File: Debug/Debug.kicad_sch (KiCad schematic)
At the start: 37 parts, among them J1 Expansion_Connector, SW1 Step, SW2 PHI1/Step, SW3 Run, SW4 SI/SC, U1 74HCT04, U10 MC14495P1, U11 HDSP-7803, U12 MC14495P1, U13 HDSP-7803, U14 MC14495P1, U15 HDSP-7803, U2 74HCT74, U3 MC14495P1, U4 HDSP-7803, U5 74HCT374, U6 MC14495P1, U7 HDSP-7803, U8 MC14495P1, U9 HDSP-7803

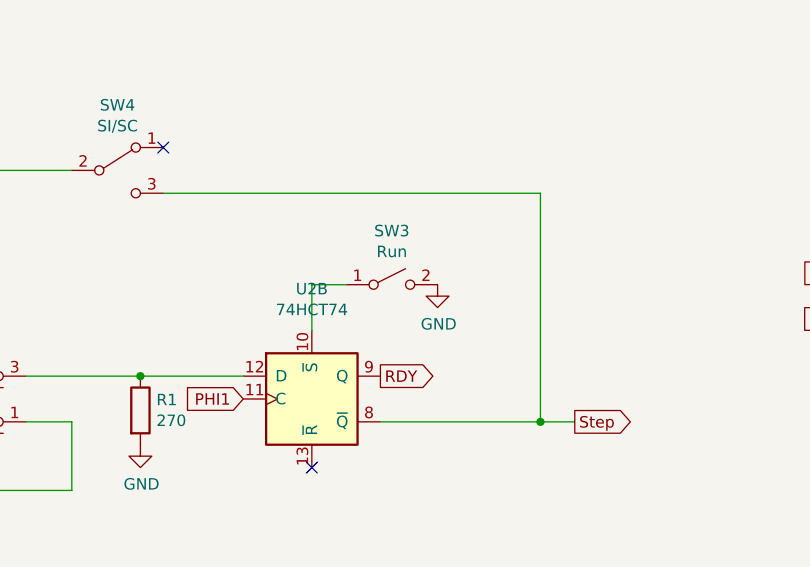
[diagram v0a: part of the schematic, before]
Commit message: Update Debug.kicad_sch
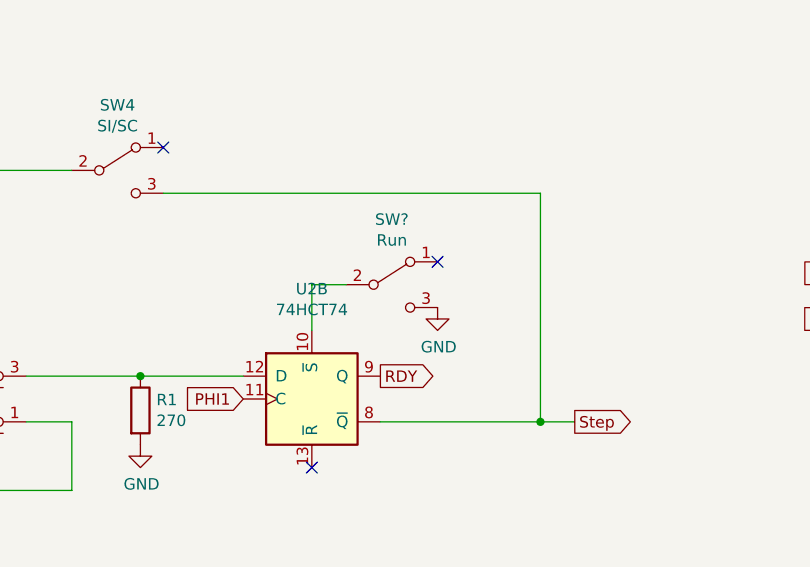
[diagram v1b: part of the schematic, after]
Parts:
- removed SW3: Run, Button_Switch_THT:SW_DIP_SPSTx01_Slide_9.78x4.72mm_W7.62mm_P2.54mm, symbol Switch:SW_SPST
- added SW?: Run, Button_Switch_THT:SW_Slide_1P2T_CK_OS102011MS2Q, symbol Switch:SW_SPDT
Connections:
- net GND: now also SW?.3 (C)
- net at U2.10 (~{S}): now also SW?.2 (B)
- no-connect marks 25 -> 26
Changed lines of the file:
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@@
   (no_connect (at 346.71 48.26))
   (no_connect (at 140.97 208.28))
+  (no_connect (at 274.32 143.51))
   (no_connect (at 233.68 46.99))
   (no_connect (at 224.79 48.26))
@@
     (pin "7")
   )
-  (symbol (lib_id "Switch:SW_SPST") (at 269.24 146.05 0) (unit 1)
-    (in_bom yes) (on_board yes)
-    (property "Reference" "SW3" (id 0) (at 269.24 140.081 0))
-    (property "Value" "Run" (id 1) (at 269.24 142.3924 0))
-    (property "Footprint" "Button_Switch_THT:SW_DIP_SPSTx01_Slide_9.78x4.72mm_W7.62mm_P2.54mm" (id 2) (at 269.24 146.05 0)
-      (effects (font (size 1.27 1.27)) hide)
-    )
-    (property "Datasheet" "~" (id 3) (at 269.24 146.05 0)
-      (effects (font (size 1.27 1.27)) hide)
-    )
-    (pin "1")
-    (pin "2")
-  )
-  (symbol (lib_id "power:GND") (at 274.32 146.05 0) (unit 1)
-    (in_bom yes) (on_board yes)
-    (property "Reference" "#PWR0104" (id 0) (at 274.32 152.4 0)
-      (effects (font (size 1.27 1.27)) hide)
-    )
-    (property "Value" "GND" (id 1) (at 274.447 150.4442 0))
-    (property "Footprint" "" (id 2) (at 274.32 146.05 0)
-      (effects (font (size 1.27 1.27)) hide)
-    )
-    (property "Datasheet" "" (id 3) (at 274.32 146.05 0)
+  (symbol (lib_id "power:GND") (at 274.32 148.59 0) (unit 1)
+    (in_bom yes) (on_board yes)
+    (property "Reference" "#PWR0104" (id 0) (at 274.32 154.94 0)
+      (effects (font (size 1.27 1.27)) hide)
+    )
+    (property "Value" "GND" (id 1) (at 274.447 152.9842 0))
+    (property "Footprint" "" (id 2) (at 274.32 148.59 0)
+      (effects (font (size 1.27 1.27)) hide)
+    )
+    (property "Datasheet" "" (id 3) (at 274.32 148.59 0)
       (effects (font (size 1.27 1.27)) hide)
     )
@@
     (pin "9")
   )
+  (symbol (lib_id "Switch:SW_SPDT") (at 269.24 146.05 0) (unit 1)
+    (in_bom yes) (on_board yes)
+    (property "Reference" "SW?" (id 0) (at 269.24 138.811 0))
+    (property "Value" "Run" (id 1) (at 269.24 141.1224 0))
+    (property "Footprint" "Button_Switch_THT:SW_Slide_1P2T_CK_OS102011MS2Q" (id 2) (at 269.24 146.05 0)
+      (effects (font (size 1.27 1.27)) hide)
+    )
+    (property "Datasheet" "~" (id 3) (at 269.24 146.05 0)
+      (effects (font (size 1.27 1.27)) hide)
+    )
+    (pin "1")
+    (pin "2")
+    (pin "3")
+  )
   (symbol (lib_id "power:GND") (at 149.86 128.27 0) (unit 1)
     (in_bom yes) (on_board yes)
@@
       (reference "SW2") (unit 1) (value "PHI1/Step") (footprint "Button_Switch_THT:SW_Slide_1P2T_CK_OS102011MS2Q")
     )
-    (path "/00000000-0000-0000-0000-000060f7634b"
-      (reference "SW3") (unit 1) (value "Run") (footprint "Button_Switch_THT:SW_DIP_SPSTx01_Slide_9.78x4.72mm_W7.62mm_P2.54mm")
-    )
     (path "/00000000-0000-0000-0000-000060f71734"
       (reference "SW4") (unit 1) (value "SI/SC") (footprint "Button_Switch_THT:SW_Slide_1P2T_CK_OS102011MS2Q")
     )
+    (path "/0aef16fa-9555-438d-87b3-458412edf5a2"
+      (reference "SW?") (unit 1) (value "Run") (footprint "Button_Switch_THT:SW_Slide_1P2T_CK_OS102011MS2Q")
+    )
     (path "/00000000-0000-0000-0000-000060f67b64"
